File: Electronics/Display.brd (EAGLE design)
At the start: 68.6 x 53.3 mm, 12 parts, among them IC1 4081N, T1 BC547, T2 BC547

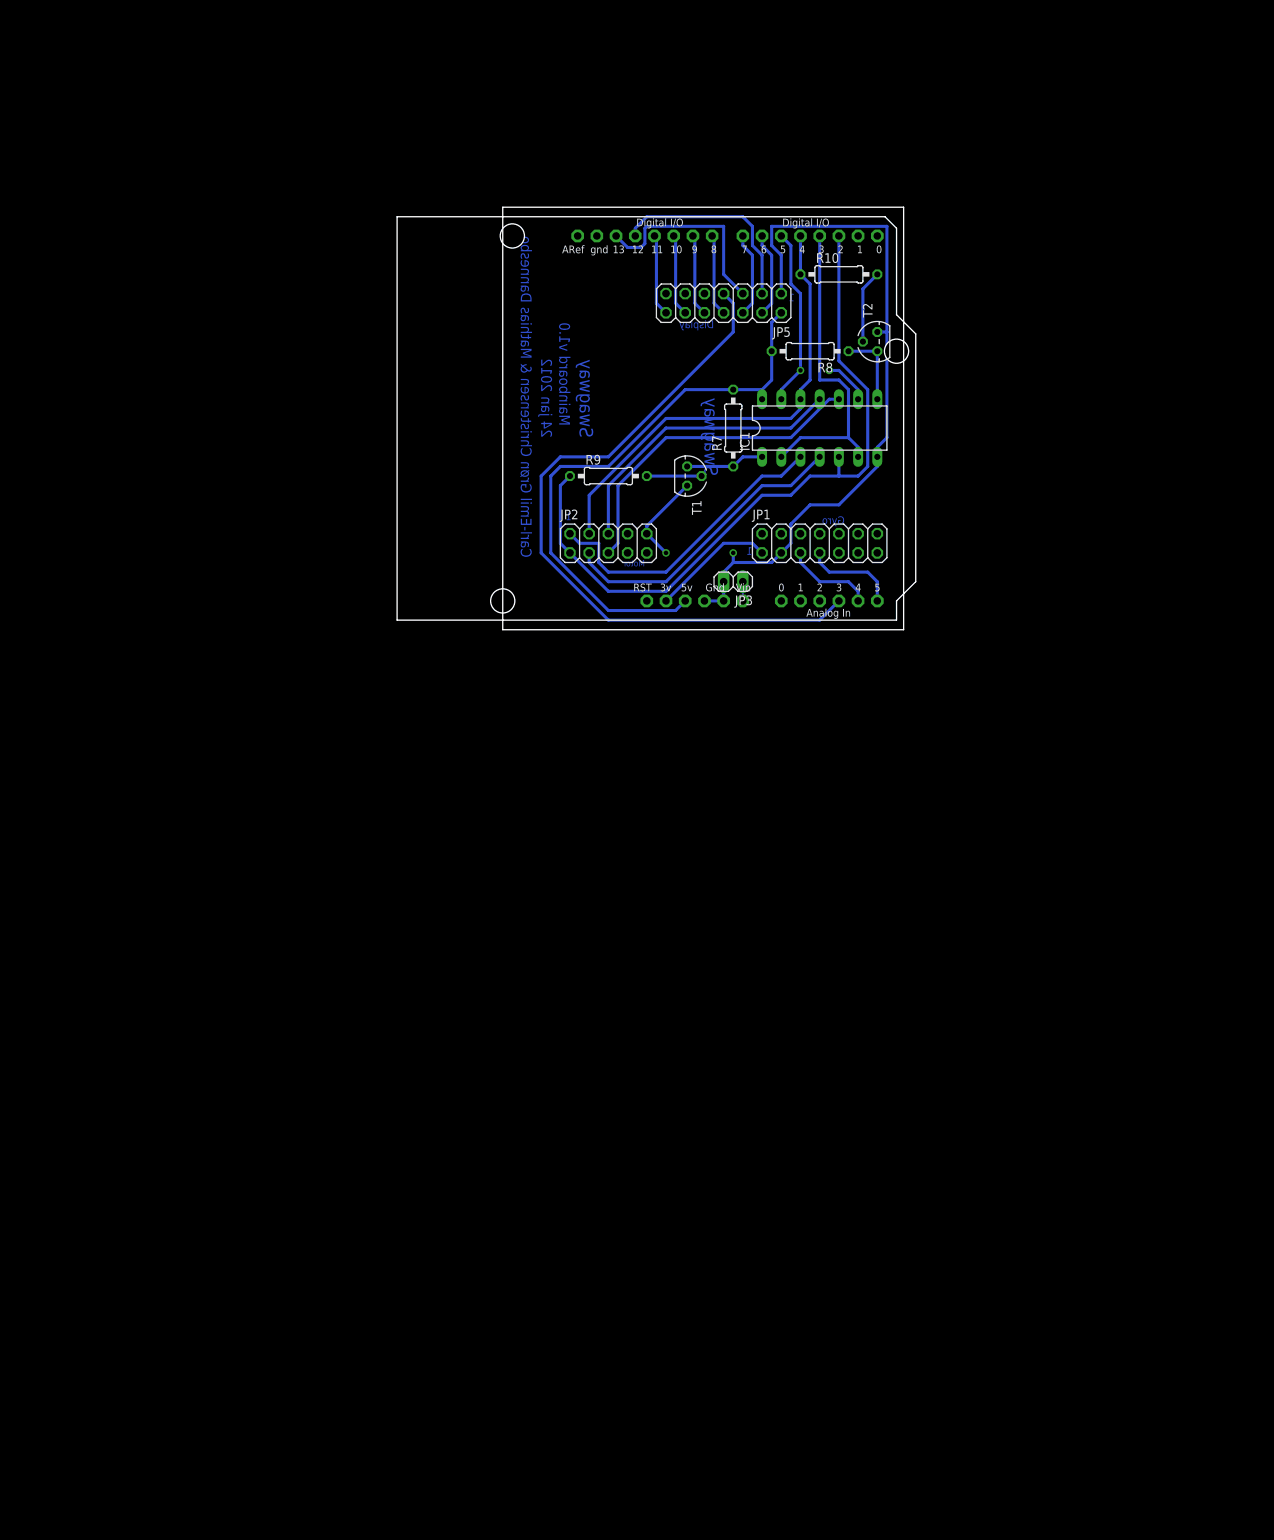
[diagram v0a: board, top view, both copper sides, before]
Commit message: 
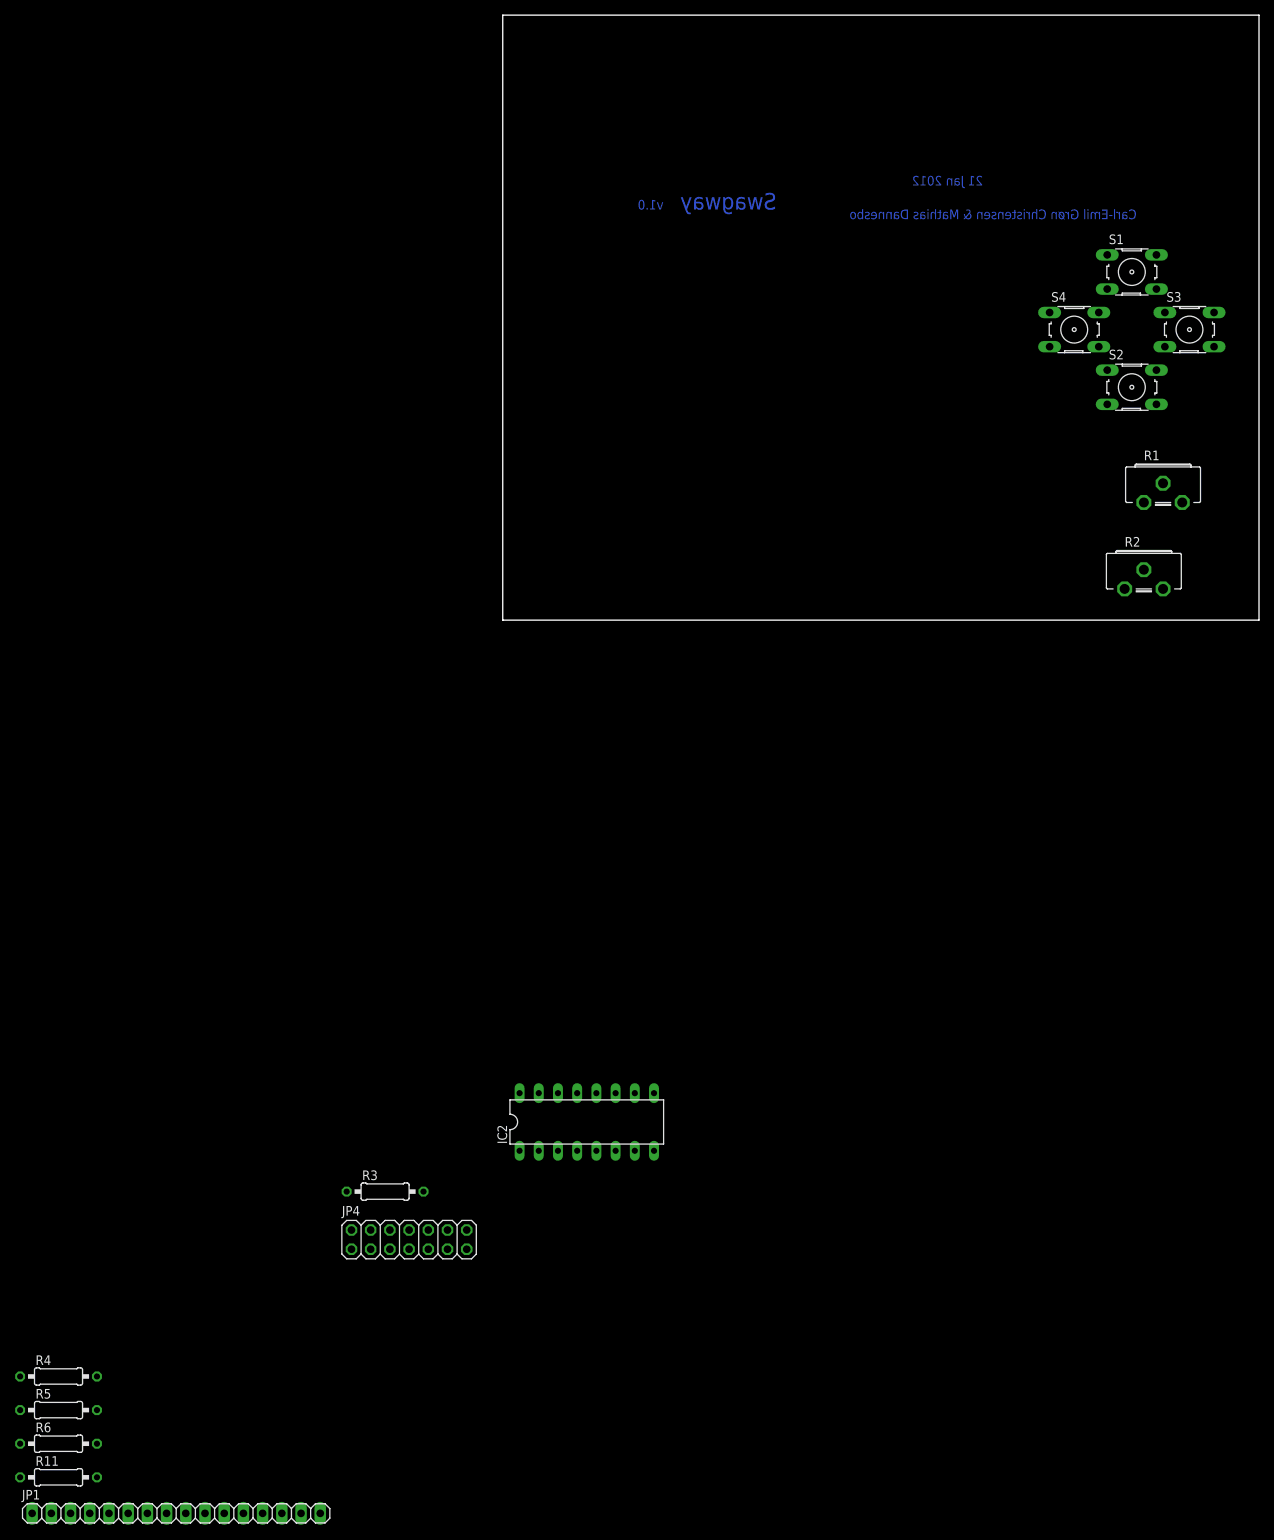
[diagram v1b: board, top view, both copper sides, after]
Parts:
- removed IC1: 4081N, 40xx:DIL14
- removed JP2: Motorcontroller, pinhead:2X05
- removed JP3: 9V Batt, pinhead:1X02
- removed JP5: Display, pinhead:2X07
- removed R10, R9: 1k, rcl:0207/10
- removed R7, R8: 10k, rcl:0207/10
- removed T1, T2: BC547, transistor:TO92
- removed U$1: ARDUINOUNO, adafruit:ARDUINO
- added IC2: 74HC165N, 74xx-eu:DIL16
- added JP4: Gyro, pinhead:2X07
- added R1: 10k, pot:CA9H
- added R11, R3, R4, R5, R6: (no value), rcl:0207/10
- added R2: (no value), pot:CA9H
- added S1, S2, S3, S4: (no value), switch-omron:B3F-10XX
- JP1: value Gyro -> (none); device pinhead:2X07 -> pinhead:1X16
- moved JP1 153.9 mm to (-43.2, -118.1)
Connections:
- removed net +3V3: JP1.1, U$1.3V
- removed net +5V: IC1.14, JP5.2, R7.2, R8.2, U$1.5V
- removed net GND: IC1.7, JP1.3, JP2.10, JP3.2, JP5.1, T1.1, T2.1, U$1.GND, U$1.GND1, U$1.GND2
- removed net N$10: IC1.5, JP2.1, R9.1, U$1.D2
- removed net N$11: IC1.2, IC1.6, U$1.D3
- removed net N$16: IC1.8, R8.1, T2.3
- removed net N$17: R9.2, T1.2
- removed net N$20: R10.2, T2.2
- removed net N$26: JP1.7, U$1.A5
- removed net N$31: JP5.4, U$1.D6
- removed net N$37: JP5.6, U$1.D7
- removed net N$38: JP5.8, U$1.D8
- removed net N$39: JP3.1, U$1.VIN
- removed net N$40: JP5.10, U$1.D9
- removed net N$41: JP1.5, U$1.A4
- removed net N$42: JP5.12, U$1.D10
- removed net N$43: JP5.14, U$1.D11
- removed net N$44: JP5.3, U$1.D12
- removed net N$45: JP5.5, U$1.D13
- removed net N$46: JP5.7, U$1.A3
- removed net N$5: IC1.11, JP2.6
- removed net N$7: IC1.13, IC1.9, U$1.D5
- removed net N$8: IC1.1, R7.1, T1.3
- new net N$12: JP1.12, R1.S
- new net N$13: IC2.9, JP4.3
- new net N$14: IC2.2, JP4.7
- new net N$15: JP1.9, JP4.6
- new net N$18: JP1.4, JP4.8
- new net N$19: JP1.3, JP4.10
- new net N$21: JP1.2, JP4.12
- new net N$22: JP1.1, JP4.14
- new net N$32: IC2.11, R4.1, S1.4
- new net N$34: IC2.12, R5.1, S2.3
- new net N$35: IC2.13, R6.1, S3.4
- new net N$36: IC2.14, R11.1, S4.4
- new net N$6: JP1.11, JP4.4
- new net N$9: IC2.1, JP4.5
- new net VCC: IC2.16
- net N$1: now also JP1.15, R2.S; no longer IC1.3, JP2.2
- net N$2: now also IC2.15, IC2.8, JP1.10, JP1.14, JP4.1, R1.E, R3.1, S1.2, S2.2, S3.2, S4.2; no longer IC1.4, JP2.3
- net N$3: now also JP1.13, JP4.2, R1.A, R11.2, R4.2, R5.2, R6.2; no longer IC1.12, JP2.4, R10.1, U$1.D4
- net N$4: now also R2.E, R3.2; no longer IC1.10, JP2.5
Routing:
- net GND: track 105.6 -> 0.00 mm
- net N$10: track 94.1 -> 0.00 mm
- net N$46: track 93.2 -> 0.00 mm
- net +5V: track 76.8 -> 0.00 mm
- net N$3: track 61.7 -> 0.00 mm
- net N$4: track 43.4 -> 0.00 mm
- net N$11: track 42.7 -> 0.00 mm
- net N$1: track 40.4 -> 0.00 mm
- net N$2: track 39.6 -> 0.00 mm
- net N$5: track 39.0 -> 0.00 mm
- net N$7: track 29.8 -> 0.00 mm, vias 1 -> 0
- net N$45: track 27.1 -> 0.00 mm
- net N$44: track 27.1 -> 0.00 mm
- net +3V3: track 16.4 -> 0.00 mm
- net N$26: track 12.5 -> 0.00 mm
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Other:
- board size 68.6 x 53.3 mm -> 100 x 80 mm
- board text added: "21 Jan 2012"
- board text added: "v1.0"
- board text removed: "1"
- board text removed: "24 jan 2012"
- board text removed: "Display"
- board text removed: "Gyro"
- board text removed: "Mainboard v1.0"
- board text removed: "Motor"
